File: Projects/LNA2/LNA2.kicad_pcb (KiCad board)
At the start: 2 copper layers, 26.9 x 47.9 mm, 14 parts, among them J1 SMA-J-P-H-ST-EM1, J2 SMA-J-P-H-ST-EM1, J3 Barrel_Jack_MountingPin, U1 TRF37A73, U2 TPS7A0533PDBV

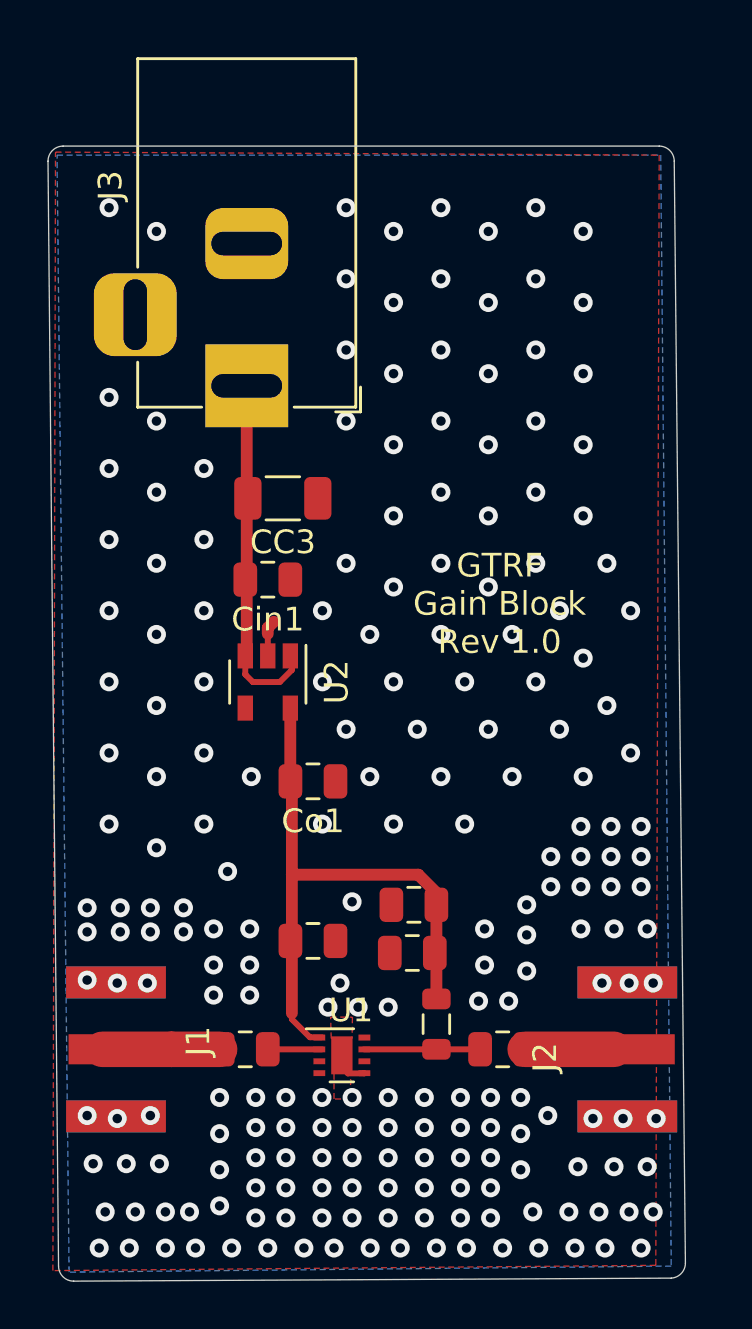
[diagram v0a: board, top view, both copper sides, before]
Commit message: post board review they are all ready to order
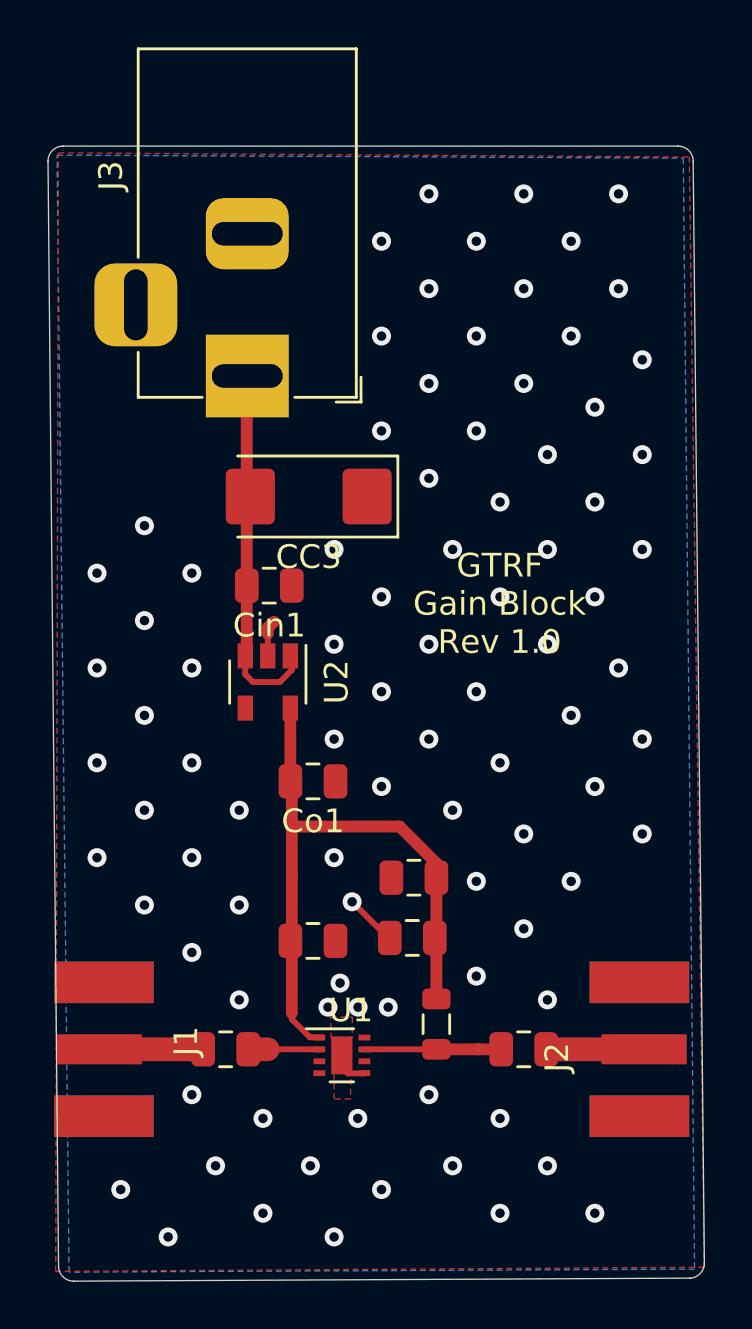
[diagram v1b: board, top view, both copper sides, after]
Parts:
- CC3: footprint Capacitor_SMD:C_1206_3216Metric -> Capacitor_Tantalum_SMD:CP_EIA-6032-28_Kemet-C
- J1, J2: footprint SAMTEC_SMA-J-P-H-ST-EM1 -> AdditionalLibs:SAMTEC_SMA-J-P-H-ST-EM1
- moved CRF2 1.14 mm to (105.2, 73.0)
- moved CC3 1.09 mm to (100.8, 56.9)
- moved CC2 0.89 mm to (109.9, 80.3)
- moved CC1 0.83 mm to (97.3, 80.3)
- moved CRF1 0.64 mm to (105.2, 75.6)
- moved J1 0.51 mm to (91.9, 80.3)
- moved J2 0.51 mm to (114.9, 80.3)
- moved J3 0.41 mm to (98.2, 51.9)
- moved Cin1 0.26 mm to (99.1, 60.7)
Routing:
- net GND: track 2.88 -> 5.10 mm, vias 215 -> 90
- net Net-(CC2-Pad1): track 3.75 -> 5.02 mm
- net Net-(CC2-Pad2): track 4.55 -> 5.57 mm
- net Net-(CDC1-Pad1): track 26.1 -> 27.0 mm
- net Net-(CC1-Pad1): track 2.29 -> 3.05 mm
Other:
- board size 26.9 x 47.9 mm -> 27.7 x 47.9 mm
